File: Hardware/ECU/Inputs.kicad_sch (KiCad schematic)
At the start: 41 parts, among them J4 EBC05DRXN, SW5 SW_DPDT_x2, U11 KP234, U12 LMV324LIDT, U13 SP720

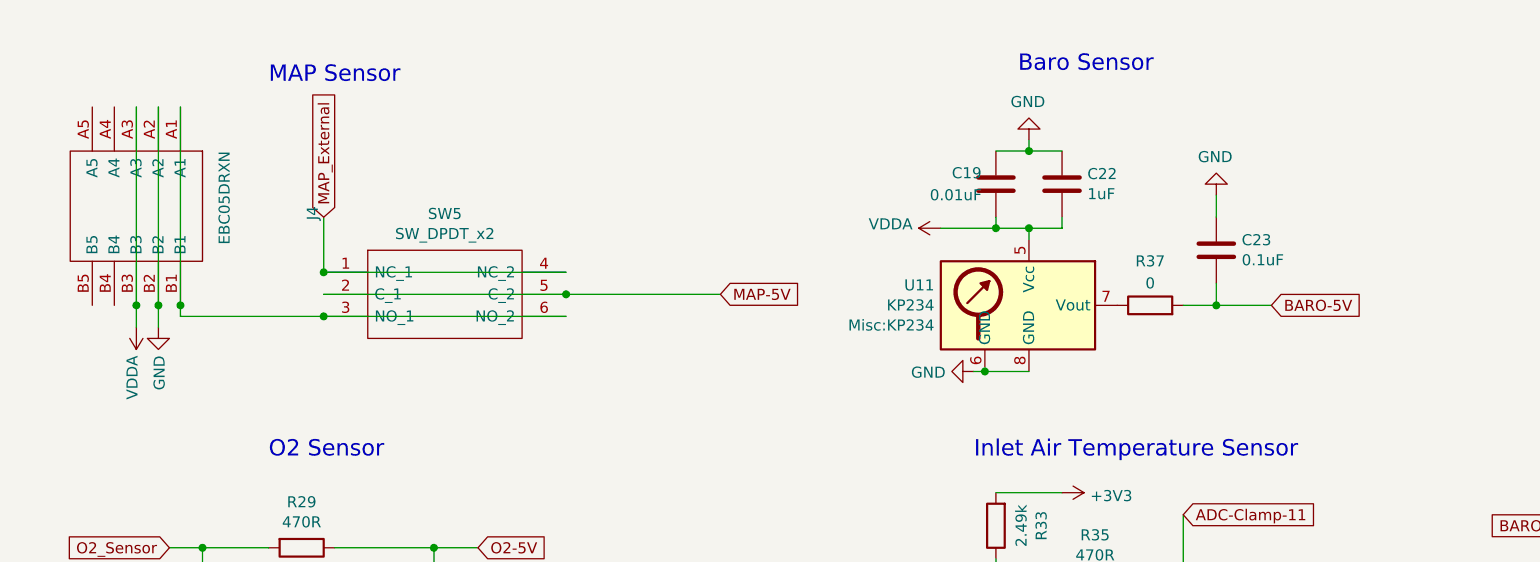
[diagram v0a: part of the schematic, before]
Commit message: PCB
Platine Vernetzt
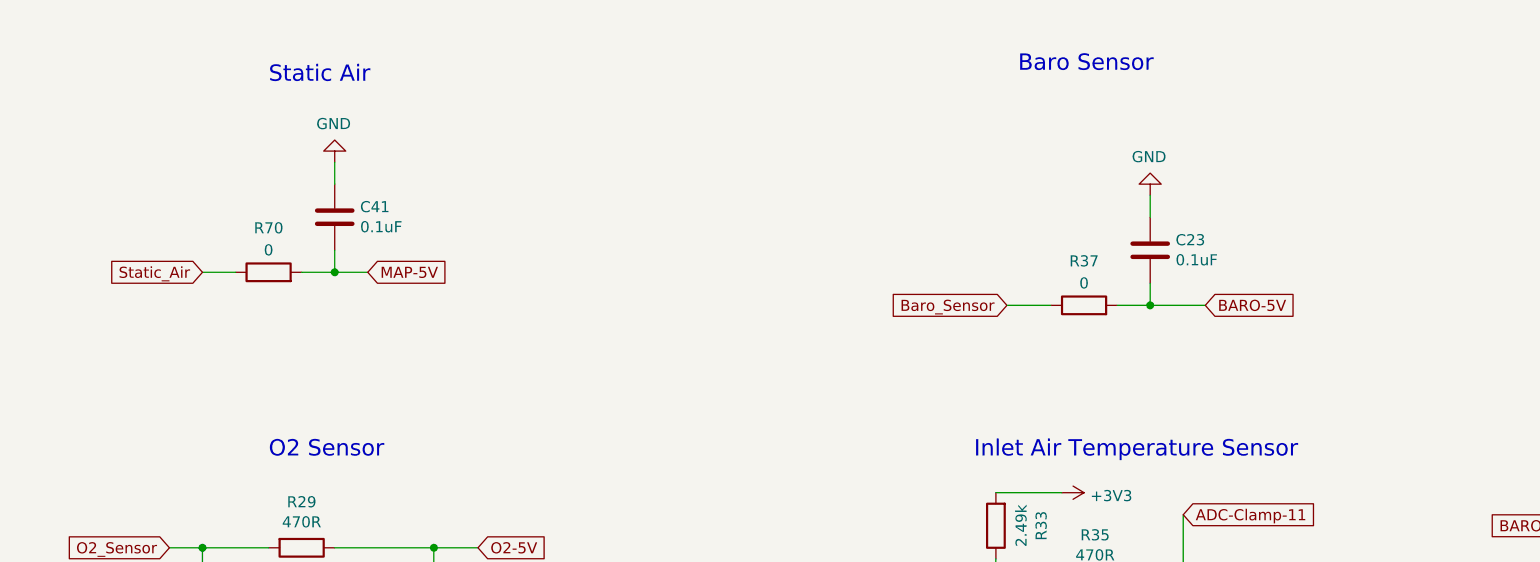
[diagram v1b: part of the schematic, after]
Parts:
- removed C19: 0.01uF, Capacitor_SMD:C_0805_2012Metric, symbol Device:C
- removed C22: 1uF, Capacitor_SMD:C_0805_2012Metric, symbol Device:C
- removed J4: EBC05DRXN, Misc:EBC05DRXN, symbol Misc:EBC05DRXN
- removed SW5: SW_DPDT_x2, Misc:AYZ0202AGRLC, symbol Misc:AYZ0202AGRLC
- removed U11: KP234, Misc:KP234, symbol Misc:KP234
- added C41: 0.1uF, Capacitor_SMD:C_0805_2012Metric, symbol Device:C
- added R70: 0, Resistor_SMD:R_0805_2012Metric, symbol Device:R
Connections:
- net GND: now also C41.1
- net MAP-5V: now also C41.2, R70.2
- net Baro_Sensor: now reaches R37.1
- new net Static_Air: R70.1
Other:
- note added: "Static Air"
- note removed: "MAP Sensor"
- moved on the sheet: C23, R37
